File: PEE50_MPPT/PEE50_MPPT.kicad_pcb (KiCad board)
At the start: 2 copper layers, 100 x 100 mm, 172 parts, among them J1 Vout, J2 Conn_01x02_Female, J3 Conn_01x02_Female, J4 Conn_01x03_Female, J5 PV_IN1, J6 PV_IN1, J7 PV_IN1, J8 PV_IN1, Q1 BC547, Q2 BC547, Q3 BC547, Q4 BC547, U1 LM3480-3.3, U10 NTA4151PT1G, U11 CSD18514Q5A, U12 CSD18543Q3A, U13 TPS552882QRPMRQ1, U14 MAX44284FAUT+T, U15 MAX44284FAUT+T, U16 NTA4151PT1G, U17 CSD18514Q5A, U18 CSD18543Q3A, U19 TPS552882QRPMRQ1, U2 MSP430FR2353TDBT, U20 MAX44284FAUT+T, U21 MAX44284FAUT+T, U22 NTA4151PT1G, U23 CSD18514Q5A, U24 CSD18543Q3A, U25 TPS552882QRPMRQ1, U26 MAX44284FAUT+T, U27 MAX44284FAUT+T, U3 ADG706BRUZ, U4 NTA4151PT1G, U5 CSD18514Q5A, U6 CSD18543Q3A, U7 TPS552882QRPMRQ1, U8 MAX44284FAUT+T, U9 MAX44284FAUT+T

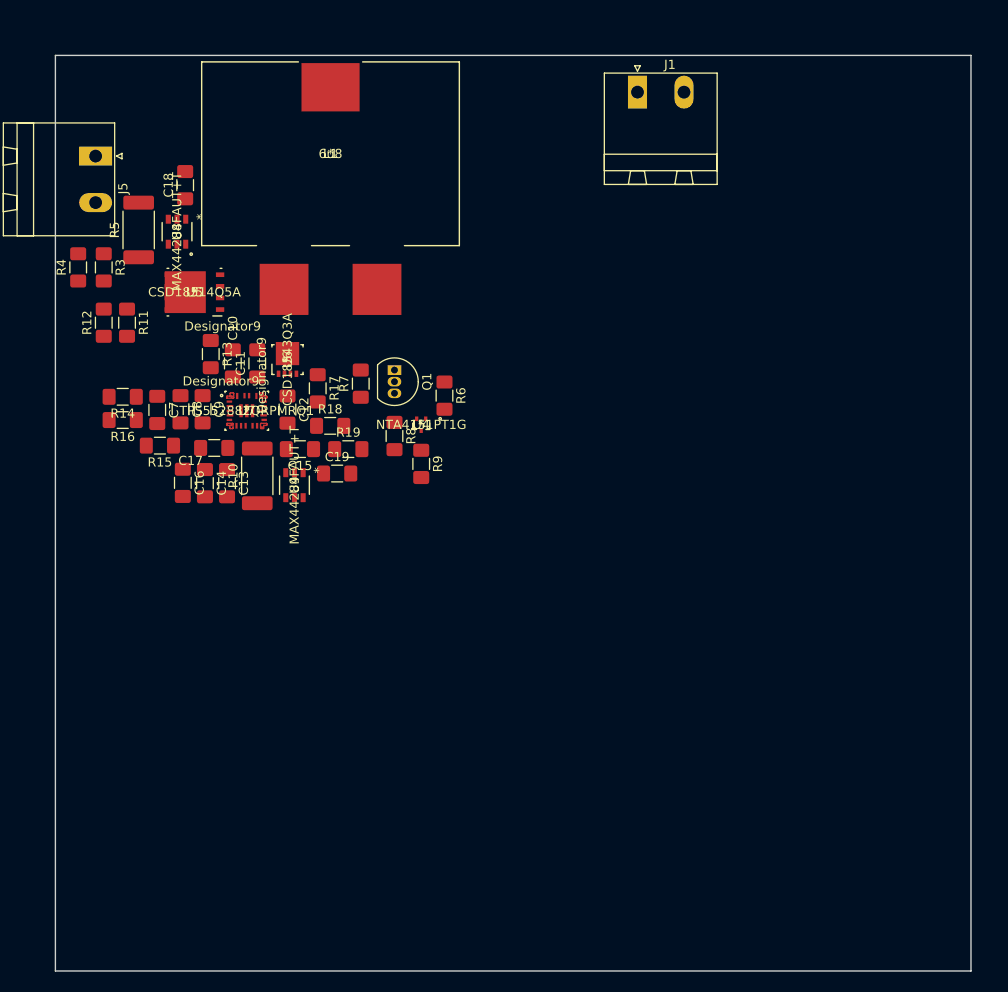
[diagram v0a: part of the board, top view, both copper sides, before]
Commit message: 1e mppt klaar (nog een keer)
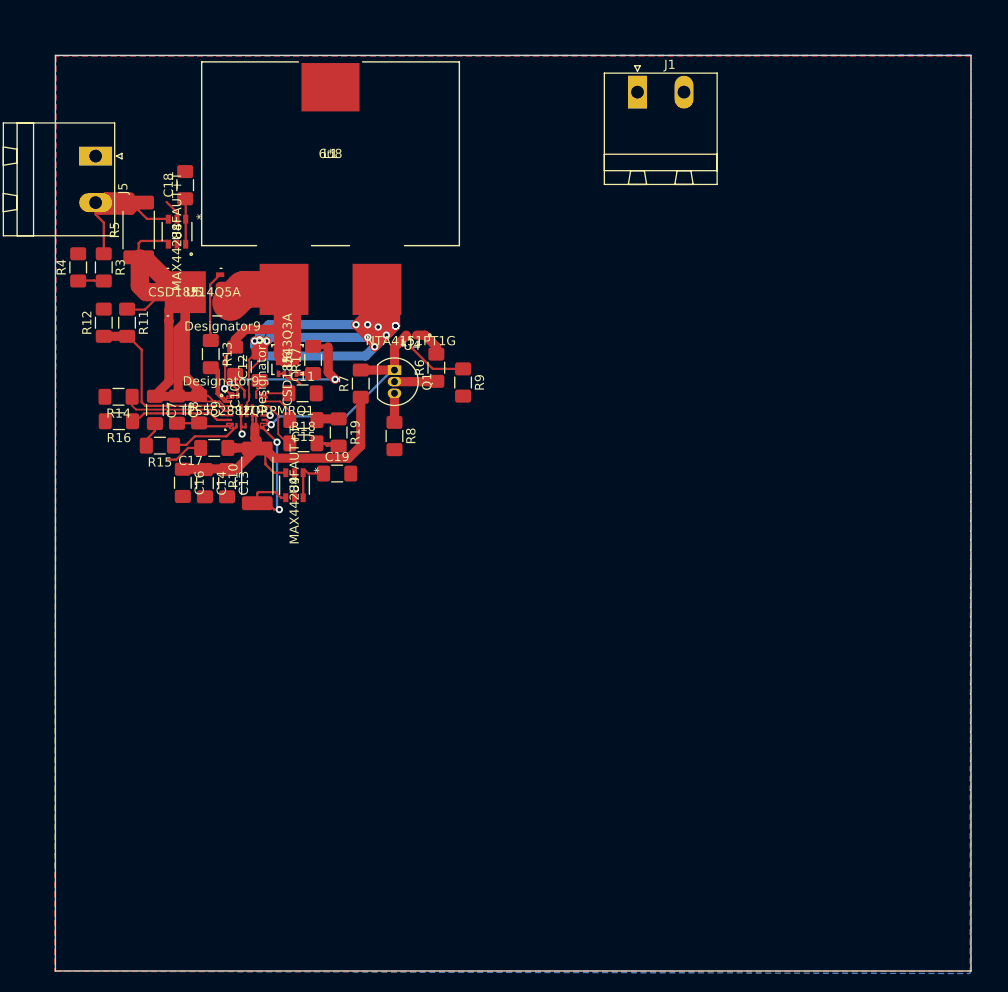
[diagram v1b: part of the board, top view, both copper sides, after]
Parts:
- moved R9 10.00 mm to (144.5, 135.7)
- moved U4 9.22 mm to (138.8, 131.2)
- moved C11 5.93 mm to (127.0, 136.9), turned to 0 degrees
- moved C12 5.57 mm to (122.3, 134.0), turned to 90 degrees
- moved R18 3.49 mm to (127.1, 142.4)
- moved C15 3.20 mm to (127.1, 139.8)
- moved R6 3.18 mm to (141.6, 134.1), turned to 90 degrees
- moved R17 3.14 mm to (128.1, 133.3), turned to 90 degrees
- moved R19 2.10 mm to (130.9, 141.2), turned to 270 degrees
- moved R14 0.45 mm to (106.9, 137.3)
- moved R16 0.44 mm to (106.9, 140.0)
- moved C10 0.39 mm to (119.6, 133.3), turned to 270 degrees
- moved C8 0.38 mm to (113.3, 138.7)
- moved C9 0.38 mm to (115.7, 138.6)
- moved C7 0.25 mm to (110.9, 138.7)
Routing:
- net Net-(C12-Pad2): track 0.00 -> 94.7 mm, vias 0 -> 14
- net /Sheet609B465C/sheet609C6964/PVin+: track 0.00 -> 69.2 mm
- net /Sheet609B465C/sheet609C6964/ISP: track 0.00 -> 39.9 mm
- net Net-(C10-Pad1): track 0.00 -> 29.8 mm
- net /Sheet609B465C/sheet609C6964/FB: track 0.00 -> 28.8 mm, vias 0 -> 1
- net Pgnd: track 0.00 -> 27.1 mm, vias 0 -> 2
- net /Sheet609B465C/sheet609C6965/R+: track 0.00 -> 24.0 mm
- net Net-(R11-Pad2): track 0.00 -> 23.4 mm
- net Net-(R17-Pad2): track 0.00 -> 19.3 mm, vias 0 -> 2
- net /Sheet609B465C/Vout: track 0.00 -> 15.6 mm, vias 0 -> 2
- net Net-(R14-Pad1): track 0.00 -> 11.9 mm
- net Net-(R16-Pad1): track 0.00 -> 10.3 mm
- net +3V3: track 0.00 -> 9.80 mm
- net Net-(R13-Pad2): track 0.00 -> 9.11 mm
- net Net-(R13-Pad1): track 0.00 -> 7.48 mm
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- added copper zone on B.Cu, net Pgnd
- added copper zone on F.Cu, net Pgnd
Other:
- net class power: clearance 0.2 -> 0.1; trace_width 0.5 -> 0.25
